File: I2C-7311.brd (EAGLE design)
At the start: 106 x 100 mm, 79 parts, among them IC1 MAX7311, Q0 P-FET, Q1 P-FET, Q10 P-FET, Q11 P-FET, Q12 P-FET, Q13 P-FET, Q14 P-FET, Q15 P-FET, Q2 P-FET, Q3 P-FET, Q4 P-FET, Q5 P-FET, Q6 P-FET, Q7 P-FET, Q8 P-FET, Q9 P-FET, SW1 A0, SW2 A1, SW3 A2

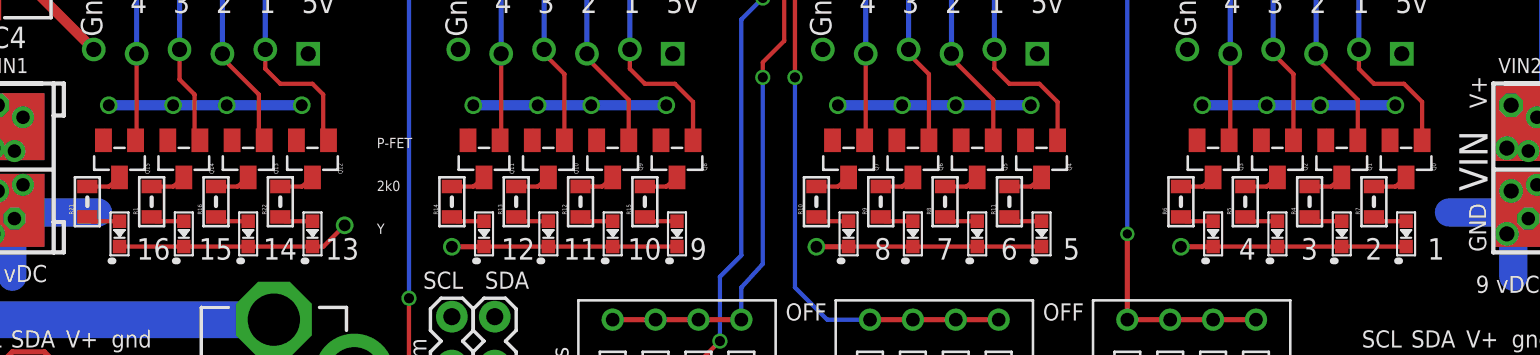
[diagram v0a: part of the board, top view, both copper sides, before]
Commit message: V3.1 again
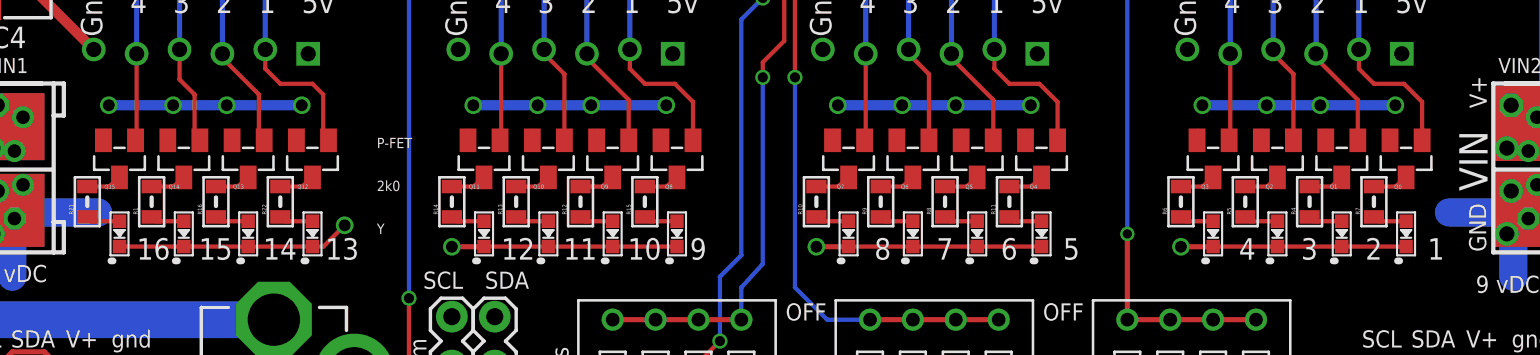
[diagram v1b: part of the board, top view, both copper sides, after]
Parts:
- turned Q0 to 90 degrees
- turned Q1 to 90 degrees
- turned Q10 to 90 degrees
- turned Q11 to 90 degrees
- turned Q12 to 90 degrees
- turned Q13 to 90 degrees
- turned Q14 to 90 degrees
- turned Q15 to 90 degrees
- turned Q2 to 90 degrees
- turned Q3 to 90 degrees
- turned Q4 to 90 degrees
- turned Q5 to 90 degrees
- turned Q6 to 90 degrees
- turned Q7 to 90 degrees
- turned Q8 to 90 degrees
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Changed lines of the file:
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@@
 <grid distance="50" unitdist="mil" unit="mil" style="dots" multiple="2" display="yes" altdistance="25" altunitdist="mil" altunit="mil"/>
 <layers>
-<layer number="1" name="Top" color="4" fill="1" visible="yes" active="yes"/>
-<layer number="16" name="Bottom" color="2" fill="1" visible="yes" active="yes"/>
+<layer number="1" name="Top" color="4" fill="1" visible="no" active="yes"/>
+<layer number="16" name="Bottom" color="2" fill="1" visible="no" active="yes"/>
 <layer number="17" name="Pads" color="23" fill="1" visible="yes" active="yes"/>
 <layer number="18" name="Vias" color="29" fill="1" visible="yes" active="yes"/>
@@
 <element name="LED3" library="SPCoast" package="0603-LED" value="Y" x="81.28" y="34.29" smashed="yes" rot="R90"/>
 <element name="LED4" library="SPCoast" package="0603-LED" value="Y" x="77.47" y="34.29" smashed="yes" rot="R90"/>
-<element name="Q0" library="SPCoast" package="SOT23" value="P-FET" x="88.9" y="38.735" smashed="yes" rot="R180">
-<attribute name="NAME" x="90.424" y="38.481" size="0.254" layer="25" ratio="11" rot="R270"/>
-</element>
-<element name="Q1" library="SPCoast" package="SOT23" value="P-FET" x="85.09" y="38.735" smashed="yes" rot="R180">
-<attribute name="NAME" x="86.614" y="38.481" size="0.254" layer="25" ratio="11" rot="R270"/>
-</element>
-<element name="Q2" library="SPCoast" package="SOT23" value="P-FET" x="81.28" y="38.735" smashed="yes" rot="R180">
-<attribute name="NAME" x="82.804" y="38.481" size="0.254" layer="25" ratio="11" rot="R270"/>
-</element>
-<element name="Q3" library="SPCoast" package="SOT23" value="P-FET" x="77.47" y="38.735" smashed="yes" rot="R180">
-<attribute name="NAME" x="78.994" y="38.481" size="0.254" layer="25" ratio="11" rot="R270"/>
+<element name="Q0" library="SPCoast" package="SOT23" value="P-FET" x="88.9" y="38.735" smashed="yes" rot="R90">
+<attribute name="NAME" x="88.646" y="37.211" size="0.254" layer="25" ratio="11" rot="R180"/>
+</element>
+<element name="Q1" library="SPCoast" package="SOT23" value="P-FET" x="85.09" y="38.735" smashed="yes" rot="R90">
+<attribute name="NAME" x="84.836" y="37.211" size="0.254" layer="25" ratio="11" rot="R180"/>
+</element>
+<element name="Q2" library="SPCoast" package="SOT23" value="P-FET" x="81.28" y="38.735" smashed="yes" rot="R90">
+<attribute name="NAME" x="81.026" y="37.211" size="0.254" layer="25" ratio="11" rot="R180"/>
+</element>
+<element name="Q3" library="SPCoast" package="SOT23" value="P-FET" x="77.47" y="38.735" smashed="yes" rot="R90">
+<attribute name="NAME" x="77.216" y="37.211" size="0.254" layer="25" ratio="11" rot="R180"/>
 </element>
 <element name="R7" library="SPCoast" package="0805-RES" value="2K0" x="86.995" y="36.195" smashed="yes" rot="R90">
@@
 <element name="LED6" library="SPCoast" package="0603-LED" value="Y" x="59.69" y="34.29" smashed="yes" rot="R90"/>
 <element name="LED7" library="SPCoast" package="0603-LED" value="Y" x="55.88" y="34.29" smashed="yes" rot="R90"/>
-<element name="Q4" library="SPCoast" package="SOT23" value="P-FET" x="67.31" y="38.735" smashed="yes" rot="R180">
-<attribute name="NAME" x="68.834" y="38.481" size="0.254" layer="25" ratio="11" rot="R270"/>
-</element>
-<element name="Q5" library="SPCoast" package="SOT23" value="P-FET" x="63.5" y="38.735" smashed="yes" rot="R180">
-<attribute name="NAME" x="65.024" y="38.481" size="0.254" layer="25" ratio="11" rot="R270"/>
-</element>
-<element name="Q6" library="SPCoast" package="SOT23" value="P-FET" x="59.69" y="38.735" smashed="yes" rot="R180">
-<attribute name="NAME" x="61.214" y="38.481" size="0.254" layer="25" ratio="11" rot="R270"/>
-</element>
-<element name="Q7" library="SPCoast" package="SOT23" value="P-FET" x="55.88" y="38.735" smashed="yes" rot="R180">
-<attribute name="NAME" x="57.404" y="38.481" size="0.254" layer="25" ratio="11" rot="R270"/>
+<element name="Q4" library="SPCoast" package="SOT23" value="P-FET" x="67.31" y="38.735" smashed="yes" rot="R90">
+<attribute name="NAME" x="67.056" y="37.211" size="0.254" layer="25" ratio="11" rot="R180"/>
+</element>
+<element name="Q5" library="SPCoast" package="SOT23" value="P-FET" x="63.5" y="38.735" smashed="yes" rot="R90">
+<attribute name="NAME" x="63.246" y="37.211" size="0.254" layer="25" ratio="11" rot="R180"/>
+</element>
+<element name="Q6" library="SPCoast" package="SOT23" value="P-FET" x="59.69" y="38.735" smashed="yes" rot="R90">
+<attribute name="NAME" x="59.436" y="37.211" size="0.254" layer="25" ratio="11" rot="R180"/>
+</element>
+<element name="Q7" library="SPCoast" package="SOT23" value="P-FET" x="55.88" y="38.735" smashed="yes" rot="R90">
+<attribute name="NAME" x="55.626" y="37.211" size="0.254" layer="25" ratio="11" rot="R180"/>
 </element>
 <element name="R11" library="SPCoast" package="0805-RES" value="2K0" x="65.405" y="36.195" smashed="yes" rot="R90">
@@
 </element>
 <element name="LED11" library="SPCoast" package="0603-LED" value="Y" x="34.29" y="34.29" smashed="yes" rot="R90"/>
-<element name="Q8" library="SPCoast" package="SOT23" value="P-FET" x="45.72" y="38.735" smashed="yes" rot="R180">
-<attribute name="NAME" x="47.244" y="38.481" size="0.254" layer="25" ratio="11" rot="R270"/>
-</element>
-<element name="Q9" library="SPCoast" package="SOT23" value="P-FET" x="41.91" y="38.735" smashed="yes" rot="R180">
-<attribute name="NAME" x="43.434" y="38.481" size="0.254" layer="25" ratio="11" rot="R270"/>
-</element>
-<element name="Q10" library="SPCoast" package="SOT23" value="P-FET" x="38.1" y="38.735" smashed="yes" rot="R180">
-<attribute name="NAME" x="39.624" y="38.481" size="0.254" layer="25" ratio="11" rot="R270"/>
-</element>
-<element name="Q11" library="SPCoast" package="SOT23" value="P-FET" x="34.29" y="38.735" smashed="yes" rot="R180">
-<attribute name="NAME" x="35.814" y="38.481" size="0.254" layer="25" ratio="11" rot="R270"/>
+<element name="Q8" library="SPCoast" package="SOT23" value="P-FET" x="45.72" y="38.735" smashed="yes" rot="R90">
+<attribute name="NAME" x="45.466" y="37.211" size="0.254" layer="25" ratio="11" rot="R180"/>
+</element>
+<element name="Q9" library="SPCoast" package="SOT23" value="P-FET" x="41.91" y="38.735" smashed="yes" rot="R90">
+<attribute name="NAME" x="41.656" y="37.211" size="0.254" layer="25" ratio="11" rot="R180"/>
+</element>
+<element name="Q10" library="SPCoast" package="SOT23" value="P-FET" x="38.1" y="38.735" smashed="yes" rot="R90">
+<attribute name="NAME" x="37.846" y="37.211" size="0.254" layer="25" ratio="11" rot="R180"/>
+</element>
+<element name="Q11" library="SPCoast" package="SOT23" value="P-FET" x="34.29" y="38.735" smashed="yes" rot="R90">
+<attribute name="NAME" x="34.036" y="37.211" size="0.254" layer="25" ratio="11" rot="R180"/>
 </element>
 <element name="R15" library="SPCoast" package="0805-RES" value="2K0" x="43.815" y="36.195" smashed="yes" rot="R90">
@@
 <element name="LED14" library="SPCoast" package="0603-LED" value="Y" x="16.51" y="34.29" smashed="yes" rot="R90"/>
 <element name="LED15" library="SPCoast" package="0603-LED" value="Y" x="12.7" y="34.29" smashed="yes" rot="R90"/>
-<element name="Q12" library="SPCoast" package="SOT23" value="P-FET" x="24.13" y="38.735" smashed="yes" rot="R180">
-<attribute name="NAME" x="25.654" y="38.481" size="0.254" layer="25" ratio="11" rot="R270"/>
-</element>
-<element name="Q13" library="SPCoast" package="SOT23" value="P-FET" x="20.32" y="38.735" smashed="yes" rot="R180">
-<attribute name="NAME" x="21.844" y="38.481" size="0.254" layer="25" ratio="11" rot="R270"/>
-</element>
-<element name="Q14" library="SPCoast" package="SOT23" value="P-FET" x="16.51" y="38.735" smashed="yes" rot="R180">
-<attribute name="NAME" x="18.034" y="38.481" size="0.254" layer="25" ratio="11" rot="R270"/>
-</element>
-<element name="Q15" library="SPCoast" package="SOT23" value="P-FET" x="12.7" y="38.735" smashed="yes" rot="R180">
-<attribute name="NAME" x="14.224" y="38.481" size="0.254" layer="25" ratio="11" rot="R270"/>
+<element name="Q12" library="SPCoast" package="SOT23" value="P-FET" x="24.13" y="38.735" smashed="yes" rot="R90">
+<attribute name="NAME" x="23.876" y="37.211" size="0.254" layer="25" ratio="11" rot="R180"/>
+</element>
+<element name="Q13" library="SPCoast" package="SOT23" value="P-FET" x="20.32" y="38.735" smashed="yes" rot="R90">
+<attribute name="NAME" x="20.066" y="37.211" size="0.254" layer="25" ratio="11" rot="R180"/>
+</element>
+<element name="Q14" library="SPCoast" package="SOT23" value="P-FET" x="16.51" y="38.735" smashed="yes" rot="R90">
+<attribute name="NAME" x="16.256" y="37.211" size="0.254" layer="25" ratio="11" rot="R180"/>
+</element>
+<element name="Q15" library="SPCoast" package="SOT23" value="P-FET" x="12.7" y="38.735" smashed="yes" rot="R90">
+<attribute name="NAME" x="12.446" y="37.211" size="0.254" layer="25" ratio="11" rot="R180"/>
 </element>
 <element name="R22" library="SPCoast" package="0805-RES" value="2K0" x="22.225" y="36.195" smashed="yes" rot="R90">
